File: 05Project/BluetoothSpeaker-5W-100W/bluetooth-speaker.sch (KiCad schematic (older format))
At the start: 16 parts, among them J1 220VAC, J2 Line-in, K1 G3MB-202P, U1 PC817, U2 MOSFET-N, U3 NE555, U4 AN6884

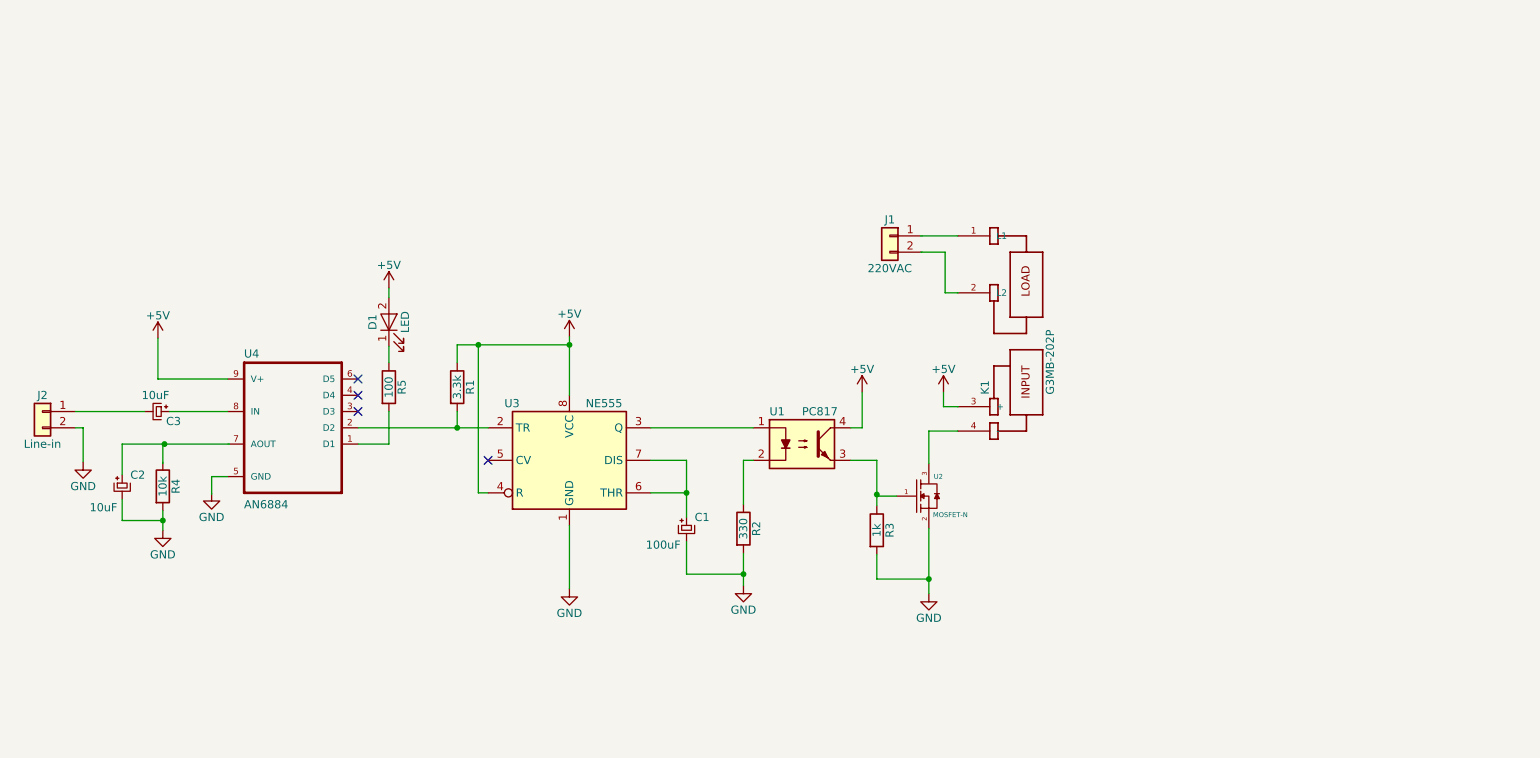
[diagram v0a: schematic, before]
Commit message: Add footprint done halt
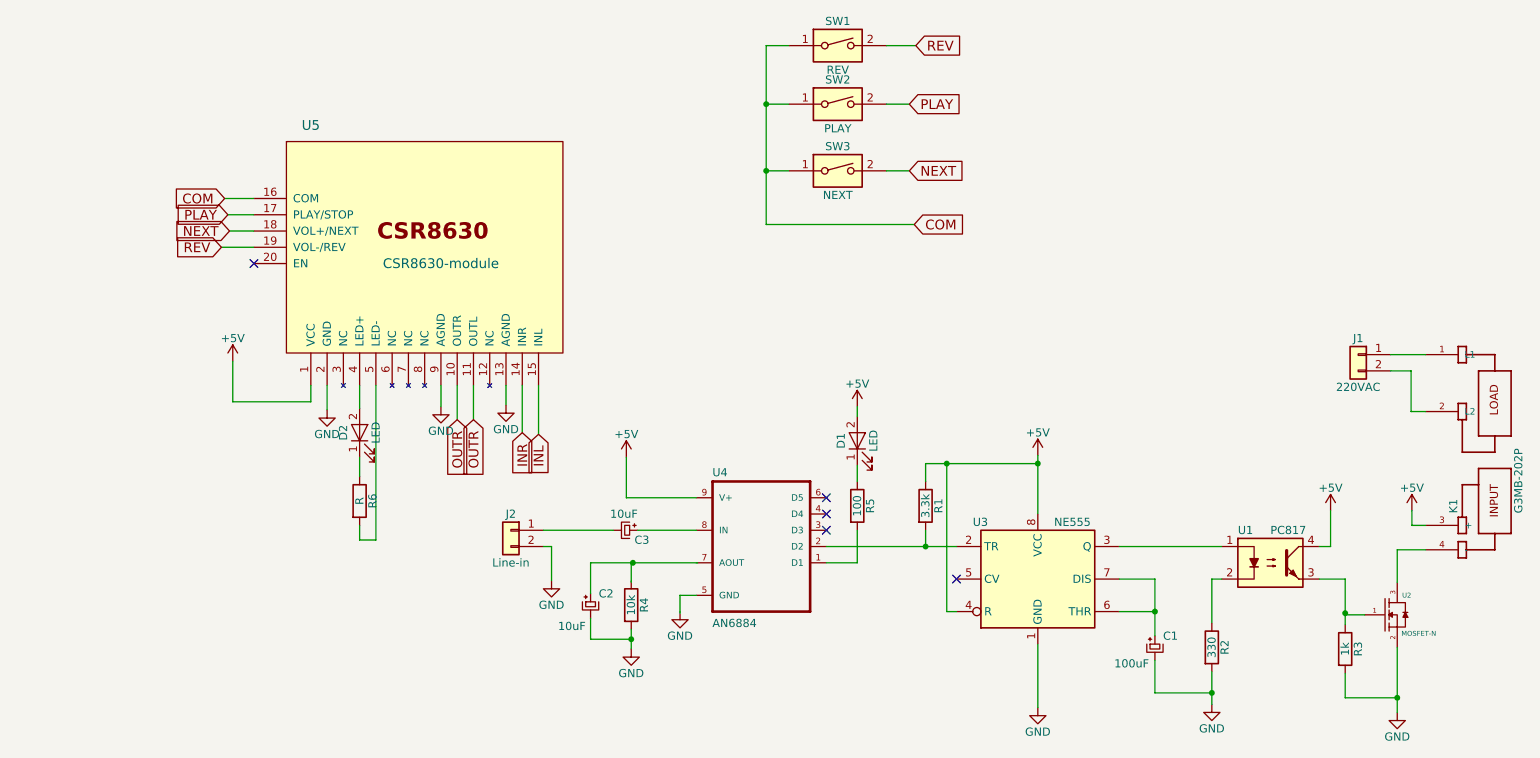
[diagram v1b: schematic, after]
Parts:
- added D2: LED, LEDs:LED_D5.0mm_FlatTop, symbol LED
- added R6: R, Resistors_SMD:R_0805_HandSoldering, symbol R
- added SW1: REV, Buttons_Switches_THT:SW_Tactile_Straight_KSA0Axx1LFTR, symbol SW_DIP_x01
- added SW2: PLAY, Buttons_Switches_THT:SW_Tactile_Straight_KSA0Axx1LFTR, symbol SW_DIP_x01
- added SW3: NEXT, Buttons_Switches_THT:SW_Tactile_Straight_KSA0Axx1LFTR, symbol SW_DIP_x01
- added U5: CSR8630-module, footprint:CSR8630-module, symbol CSR8630-module
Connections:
- net labels added: COM, INL, INR, NEXT, OUTR, PLAY, REV
- wire segments 53 -> 80
- no-connect marks 4 -> 5
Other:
- moved on the sheet: C1, C2, C3, D1, J1, J2, K1, R1, R2, R3, R4, R5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
